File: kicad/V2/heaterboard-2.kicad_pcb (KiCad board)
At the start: 4 copper layers, 12 parts, among them J1 Screw_Terminal_01x02, J2 Conn_01x05_Pin, J3 Conn_01x04_Pin, Q1 Q_NMOS_GDS, U1 LM317_TO-220

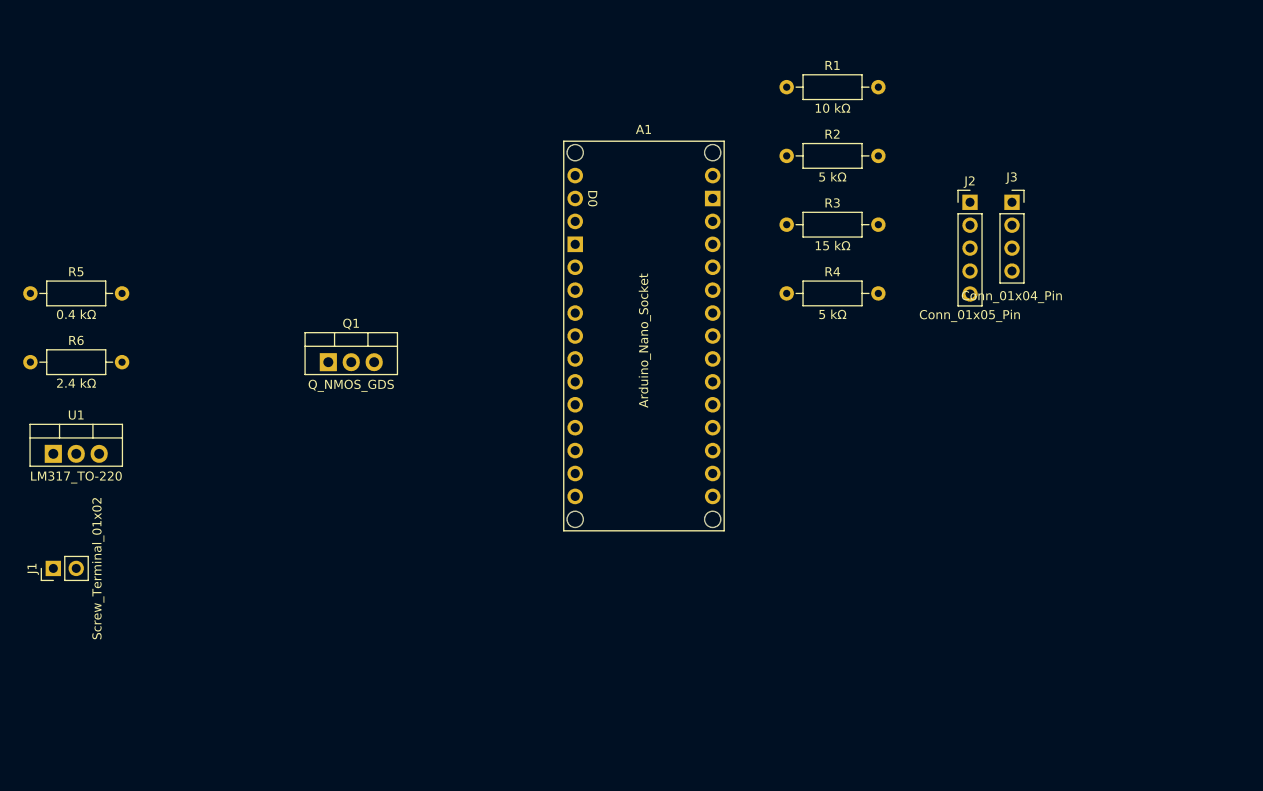
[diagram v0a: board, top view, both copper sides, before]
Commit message: pcb layout
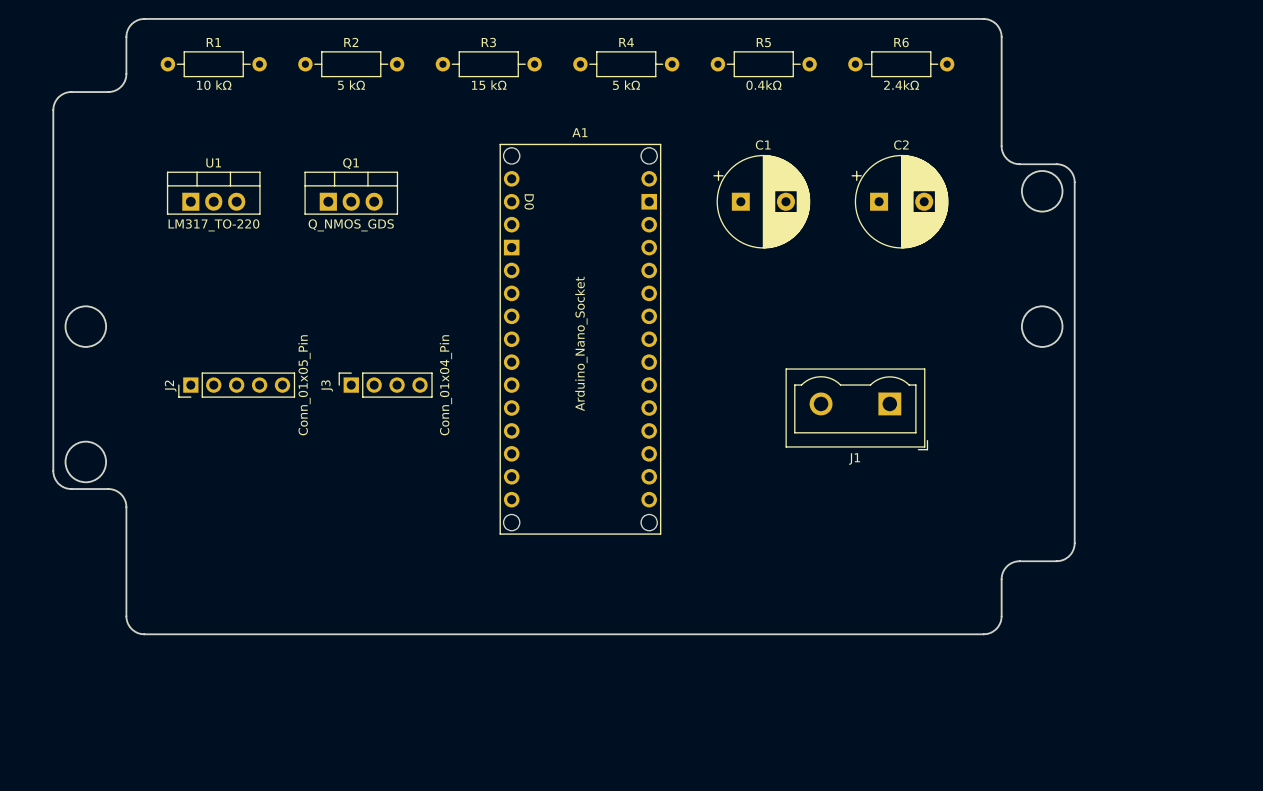
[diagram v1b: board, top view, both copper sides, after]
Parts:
- added C1: 100nF, Capacitor_THT:CP_Radial_D10.0mm_P5.00mm, F.Cu at (127.0, 61.0)
- added C2: 1μF, Capacitor_THT:CP_Radial_D10.0mm_P5.00mm, F.Cu at (142.3, 61.0)
- J1: footprint Connector_PinHeader_2.54mm:PinHeader_1x02_P2.54mm_Vertical -> TerminalBlock:TerminalBlock_Wuerth_691311400102_P7.62mm
- R5: value 0.4 kΩ -> 0.4kΩ
- R6: value 2.4 kΩ -> 2.4kΩ
- moved R6 97.2 mm to (139.7, 45.7)
- moved J1 94.5 mm to (143.5, 83.4), turned to 180 degrees
- moved J2 88.7 mm to (66.0, 81.3), turned to 90 degrees
- moved R5 80.3 mm to (124.5, 45.7)
- moved J3 76.0 mm to (83.8, 81.3), turned to 90 degrees
- moved R1 68.6 mm to (63.5, 45.7)
- moved R2 54.3 mm to (78.7, 45.7)
- moved R3 42.0 mm to (94.0, 45.7)
- moved R4 34.2 mm to (109.2, 45.7)
- moved U1 31.8 mm to (66.0, 61.0)
- moved Q1 17.8 mm to (81.3, 61.0)
- moved A1 7.05 mm to (109.2, 97.8)
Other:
- board outline added: 113.2 x 68.2 mm

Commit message: pcb layout and began routing
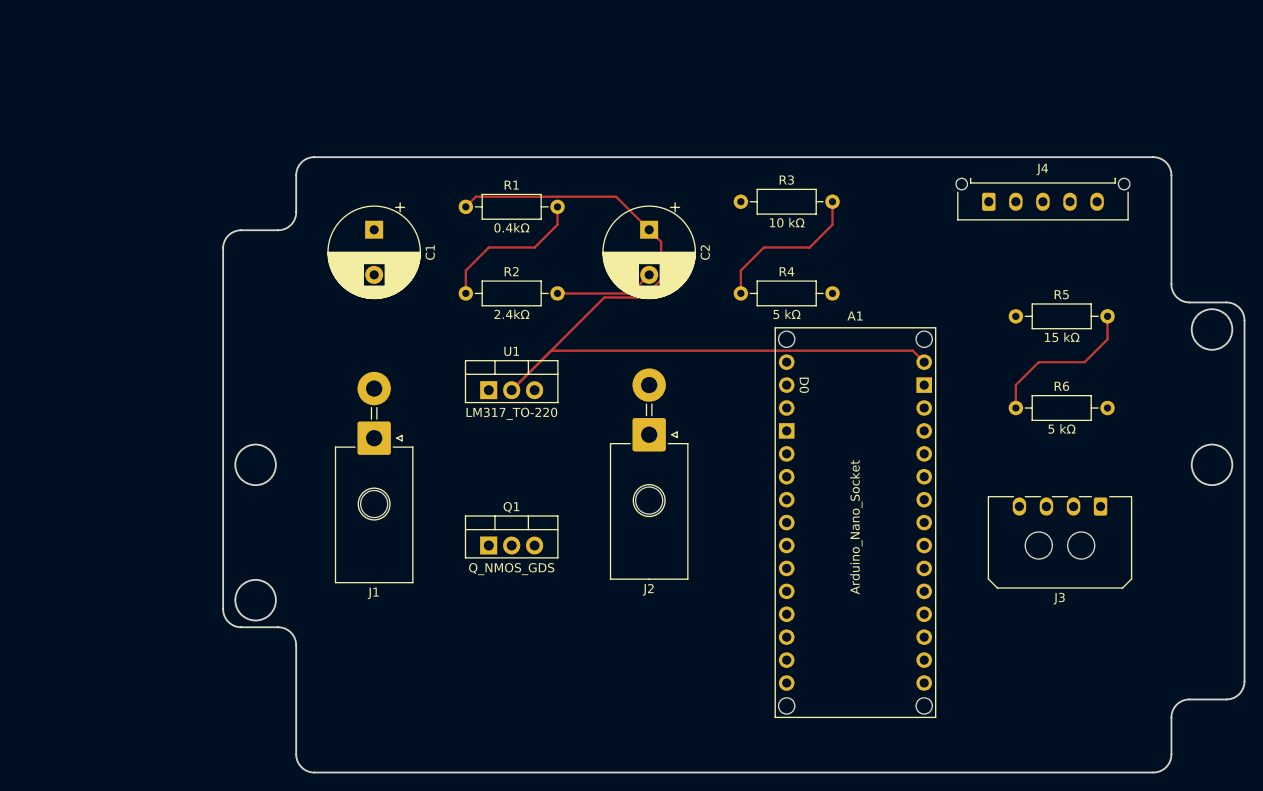
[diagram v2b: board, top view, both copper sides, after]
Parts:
- added J1: Screw_Terminal_01x02, Connector_Molex:Molex_Mega-Fit_76825-0002_2x01_P5.70mm_Horizontal, F.Cu at (86.4, 87.2)
- J2: renamed from J1; footprint TerminalBlock:TerminalBlock_Wuerth_691311400102_P7.62mm -> Connector_Molex:Molex_Mega-Fit_76825-0002_2x01_P5.70mm_Horizontal
- J3: footprint Connector_PinSocket_2.54mm:PinSocket_1x04_P2.54mm_Vertical -> Connector_Molex:Molex_Micro-Fit_3.0_43650-0400_1x04_P3.00mm_Horizontal
- J4: renamed from J2; footprint Connector_PinHeader_2.54mm:PinHeader_1x05_P2.54mm_Vertical -> Connector_Molex:Molex_Micro-Fit_3.0_43650-0515_1x05_P3.00mm_Vertical
- moved J4 90.7 mm to (154.5, 61.0), turned to 0 degrees
- moved J3 84.1 mm to (166.9, 94.7), turned to 180 degrees
- moved R5 69.4 mm to (157.5, 73.7)
- moved R3 65.3 mm to (127.0, 61.0)
- moved R6 61.5 mm to (157.5, 83.8)
- moved R4 54.5 mm to (127.0, 71.1)
- moved R2 50.1 mm to (96.5, 71.1)
- moved Q1 42.0 mm to (99.1, 99.1)
- moved C1 40.8 mm to (86.4, 64.1), turned to -90 degrees
- moved U1 39.1 mm to (99.1, 81.8)
- moved A1 36.6 mm to (139.7, 118.1)
- moved R1 32.1 mm to (96.5, 61.5)
- moved J2 26.9 mm to (116.8, 86.8)
- moved C2 25.7 mm to (116.8, 64.1), turned to -90 degrees
- renumbered R5 to R1, R6 to R2, R1 to R3, R2 to R4, R3 to R5, R4 to R6
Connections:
- R4 pad 2: unconnected-(R2---Pad2) -> GND
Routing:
- net +9V: track 0.00 -> 98.1 mm
- net /A0: track 0.00 -> 17.3 mm
- net /A1: track 0.00 -> 17.3 mm
- net Net-(R1--): track 0.00 -> 16.8 mm
- net GND: track 0.00 -> 11.0 mm
- added copper zone on In1.Cu, net (none)
- added copper zone on In2.Cu, net (none)
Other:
- outline, holes or cut-outs redrawn
